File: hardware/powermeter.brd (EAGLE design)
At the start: 97.8 x 94.9 mm, 64 parts, among them IC1 LDL112D33R, J2 TP1, J3 TP2, J6 FEMALE 2x3, U1 MCP73833T-AMI/UN, U2 ESP-WROOM-32, U3 INA219AIDR, Y1 ABM7-12.000MHZ-D2Y-T

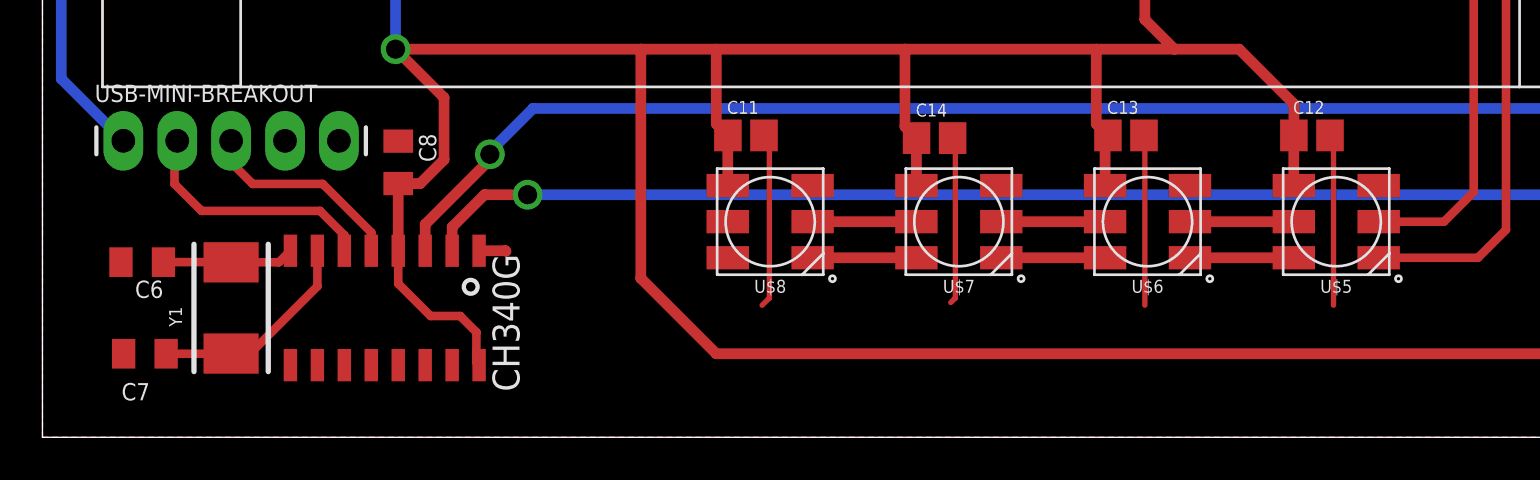
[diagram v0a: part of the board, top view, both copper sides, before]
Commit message: updated gnd plane
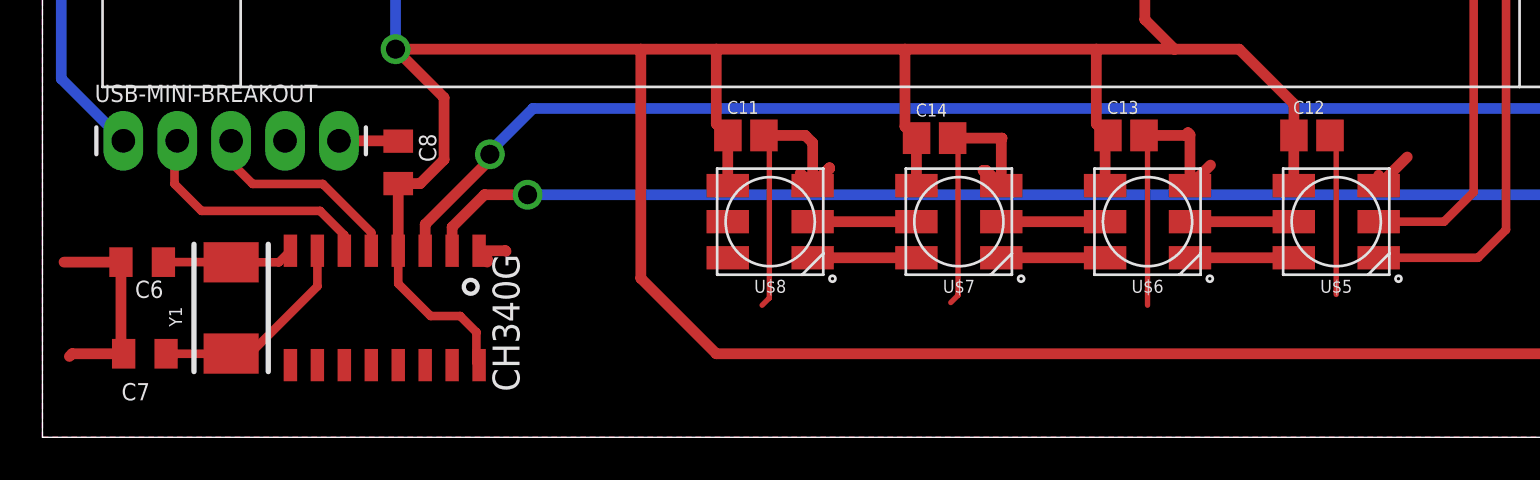
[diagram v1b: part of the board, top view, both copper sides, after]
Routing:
- net GND: track 210.5 -> 246.7 mm
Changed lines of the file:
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@@
 <wire x1="34.251" y1="13.97" x2="34.251" y2="6.565" width="0.254" layer="1"/>
 <wire x1="34.251" y1="6.565" x2="33.909" y2="6.223" width="0.254" layer="1"/>
-<wire x1="42.887" y1="14.097" x2="43.014" y2="13.97" width="0.254" layer="1"/>
-<wire x1="43.014" y1="13.97" x2="43.014" y2="6.565" width="0.254" layer="1"/>
-<wire x1="43.014" y1="6.565" x2="42.799" y2="6.35" width="0.254" layer="1"/>
-<wire x1="51.904" y1="14.224" x2="51.943" y2="14.185" width="0.254" layer="1"/>
-<wire x1="51.943" y1="14.185" x2="51.943" y2="6.223" width="0.254" layer="1"/>
-<wire x1="60.667" y1="14.224" x2="60.833" y2="14.058" width="0.254" layer="1"/>
-<wire x1="60.833" y1="14.058" x2="60.833" y2="6.223" width="0.254" layer="1"/>
+<wire x1="42.887" y1="14.097" x2="42.97" y2="14.014" width="0.254" layer="1"/>
+<wire x1="42.97" y1="14.014" x2="43.141" y2="13.843" width="0.254" layer="1"/>
+<wire x1="43.141" y1="13.843" x2="43.141" y2="6.692" width="0.254" layer="1"/>
+<wire x1="43.141" y1="6.692" x2="42.799" y2="6.35" width="0.254" layer="1"/>
+<wire x1="51.904" y1="14.224" x2="52.07" y2="14.058" width="0.254" layer="1"/>
+<wire x1="52.07" y1="14.058" x2="52.07" y2="6.223" width="0.254" layer="1"/>
+<wire x1="60.667" y1="14.224" x2="60.96" y2="13.931" width="0.254" layer="1"/>
+<wire x1="60.96" y1="13.931" x2="60.96" y2="6.731" width="0.254" layer="1"/>
 <via x="82.55" y="34.29" extent="1-16" drill="0.9"/>
 <wire x1="85.471" y1="76.6572" x2="85.471" y2="77.978" width="0.254" layer="1"/>
@@
 <wire x1="74.93" y1="77.597" x2="74.93" y2="77.47" width="0.254" layer="1"/>
 <wire x1="85.471" y1="77.978" x2="84.963" y2="78.486" width="0.254" layer="1"/>
+<wire x1="3.826" y1="3.937" x2="3.699" y2="4.064" width="0.508" layer="1"/>
+<wire x1="3.699" y1="4.064" x2="3.699" y2="8.255" width="0.508" layer="1"/>
+<wire x1="3.826" y1="3.937" x2="1.397" y2="3.937" width="0.508" layer="1"/>
+<wire x1="1.397" y1="3.937" x2="1.27" y2="3.81" width="0.508" layer="1"/>
+<wire x1="3.699" y1="8.255" x2="1.016" y2="8.255" width="0.508" layer="1"/>
+<wire x1="20.574" y1="8.791" x2="20.955" y2="8.41" width="0.508" layer="1"/>
+<wire x1="20.955" y1="8.41" x2="20.955" y2="8.255" width="0.508" layer="1"/>
+<wire x1="36.29" y1="11.86" x2="37.084" y2="12.654" width="0.508" layer="1"/>
+<wire x1="37.084" y1="12.654" x2="37.084" y2="12.7" width="0.508" layer="1"/>
+<wire x1="37.084" y1="12.7" x2="36.29" y2="11.906" width="0.508" layer="1"/>
+<wire x1="36.29" y1="11.906" x2="36.29" y2="11.86" width="0.508" layer="1"/>
+<wire x1="36.29" y1="11.86" x2="35.704" y2="12.446" width="0.508" layer="1"/>
+<wire x1="45.18" y1="11.86" x2="44.467" y2="12.573" width="0.508" layer="1"/>
+<wire x1="44.467" y1="12.573" x2="44.323" y2="12.573" width="0.508" layer="1"/>
+<wire x1="44.323" y1="12.573" x2="45.036" y2="11.86" width="0.508" layer="1"/>
+<wire x1="45.036" y1="11.86" x2="45.18" y2="11.86" width="0.508" layer="1"/>
+<wire x1="45.18" y1="11.86" x2="45.18" y2="11.906" width="0.508" layer="1"/>
+<wire x1="54.07" y1="11.86" x2="55.037" y2="12.827" width="0.508" layer="1"/>
+<wire x1="54.07" y1="11.86" x2="54.07" y2="12.224" width="0.508" layer="1"/>
+<wire x1="62.96" y1="11.86" x2="64.308" y2="13.208" width="0.508" layer="1"/>
+<wire x1="62.96" y1="11.86" x2="62.96" y2="12.351" width="0.508" layer="1"/>
+<wire x1="51.904" y1="14.224" x2="53.848" y2="14.224" width="0.508" layer="1"/>
+<wire x1="53.848" y1="14.224" x2="53.975" y2="14.351" width="0.508" layer="1"/>
+<wire x1="53.975" y1="14.351" x2="54.07" y2="14.256" width="0.508" layer="1"/>
+<wire x1="54.07" y1="14.256" x2="54.07" y2="11.86" width="0.508" layer="1"/>
+<wire x1="45.18" y1="11.86" x2="45.18" y2="14.065" width="0.508" layer="1"/>
+<wire x1="45.18" y1="14.065" x2="45.212" y2="14.097" width="0.508" layer="1"/>
+<wire x1="45.212" y1="14.097" x2="43.053" y2="14.097" width="0.508" layer="1"/>
+<wire x1="43.053" y1="14.097" x2="42.97" y2="14.014" width="0.508" layer="1"/>
+<wire x1="36.29" y1="11.86" x2="36.29" y2="13.875" width="0.508" layer="1"/>
+<wire x1="35.941" y1="14.224" x2="33.997" y2="14.224" width="0.508" layer="1"/>
+<wire x1="36.29" y1="13.875" x2="35.941" y2="14.224" width="0.508" layer="1"/>
+<wire x1="16.764" y1="13.954" x2="16.748" y2="13.97" width="0.508" layer="1"/>
+<wire x1="16.748" y1="13.97" x2="13.97" y2="13.97" width="0.508" layer="1"/>
 </signal>
 <signal name="THERM">
